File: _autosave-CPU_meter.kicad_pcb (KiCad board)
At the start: 4 copper layers, 25 parts, among them IC1 ATMEGA328P-P, SW1 SPST, U1 74HC595, U2 74HC595, U3 74HC595, U4 74HC595, U5 74HC595, U6 LM7805, Y1 16.00 MHz

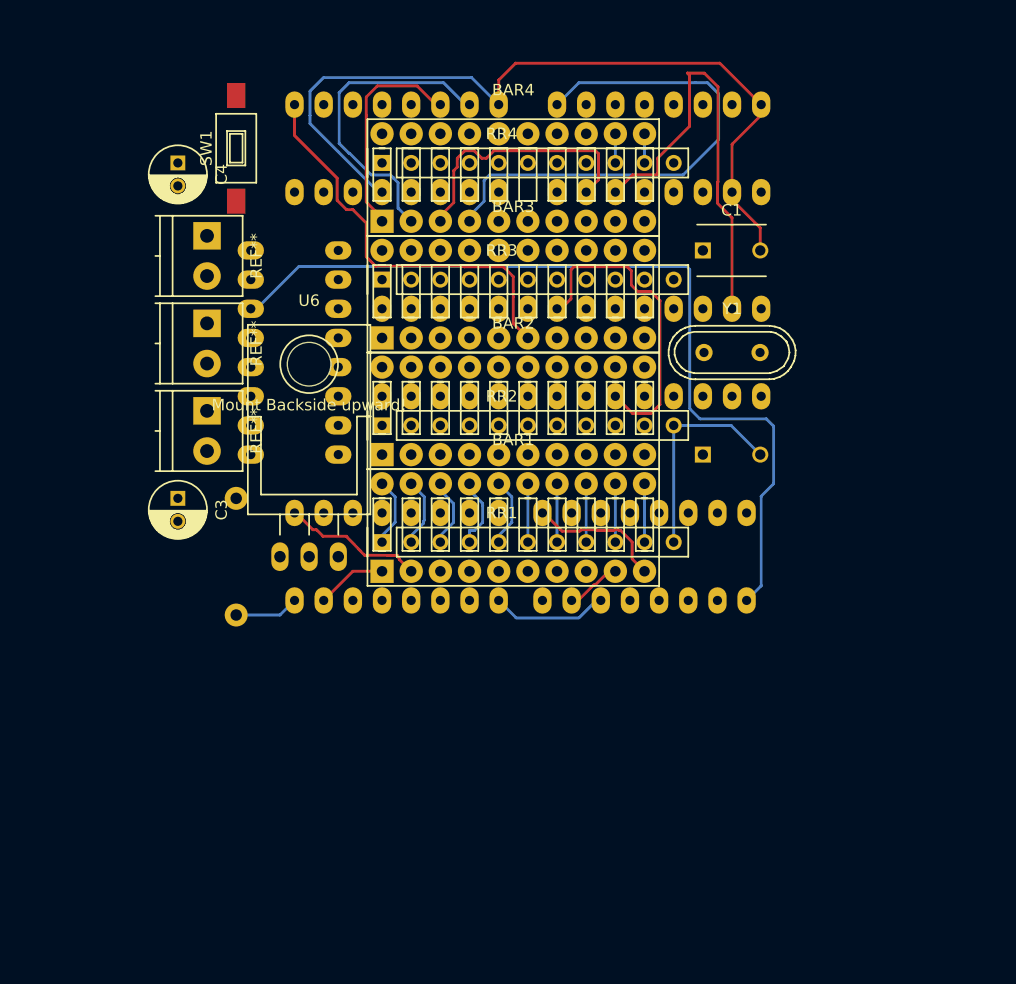
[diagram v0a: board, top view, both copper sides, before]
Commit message: PCB progress :)
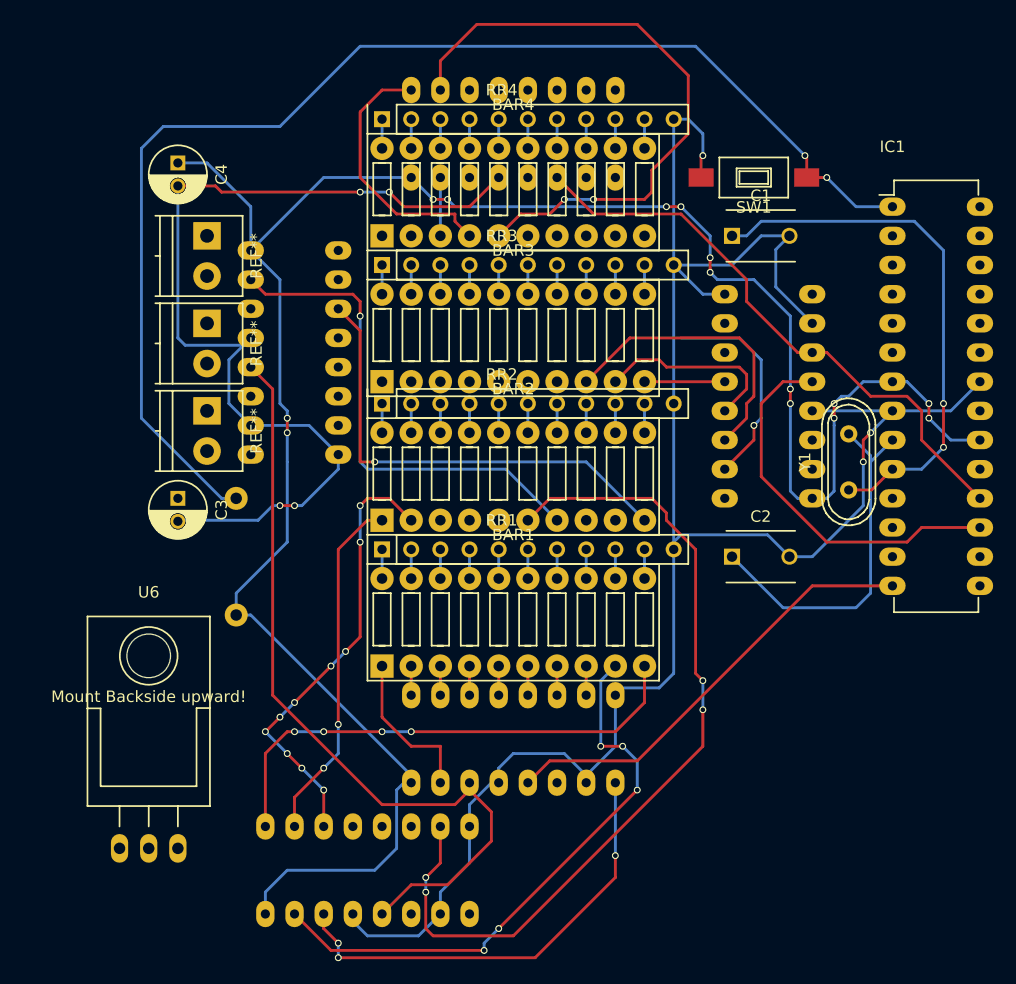
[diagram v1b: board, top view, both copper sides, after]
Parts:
- C2, IC1: moved to F.Cu
- moved U4 50.8 mm to (160.7, 147.3), turned to 0 degrees
- moved IC1 45.3 mm to (175.3, 121.9), turned to 0 degrees
- moved SW1 45.2 mm to (163.2, 119.4), turned to 180 degrees
- moved U2 36.4 mm to (120.7, 175.9)
- moved U6 29.0 mm to (110.5, 177.8)
- moved U1 18.8 mm to (133.3, 164.5)
- moved Y1 13.9 mm to (171.4, 144.1), turned to 90 degrees
- moved U5 12.8 mm to (133.3, 111.8)
- moved C2 9.25 mm to (161.3, 152.4)
- moved BAR1 8.25 mm to (142.2, 158.1)
- moved BAR2 5.72 mm to (142.2, 145.4)
- moved BAR3 3.81 mm to (142.2, 133.3)
- moved RR4 3.81 mm to (142.2, 114.3)
- moved C1 2.84 mm to (161.3, 124.5)
- moved RR2 1.91 mm to (142.2, 139.1)
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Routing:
- net GND: track 128.7 -> 258.1 mm, vias 0 -> 7
- net Net-(IC1-Pad1): track 0.00 -> 110.5 mm, vias 0 -> 2
- net Net-(IC1-Pad17): track 0.00 -> 102.5 mm
- net VCC: track 95.8 -> 189.5 mm, vias 0 -> 14
- net Net-(U2-Pad9): track 76.1 -> 0.00 mm
- net Net-(BAR2-Pad6): track 0.00 -> 75.7 mm, vias 0 -> 4
- net Net-(IC1-Pad18): track 0.00 -> 51.0 mm
- net Net-(BAR1-Pad9): track 4.86 -> 51.1 mm, vias 0 -> 5
- net Net-(BAR2-Pad7): track 0.00 -> 43.5 mm, vias 0 -> 1
- net Net-(BAR3-Pad10): track 50.2 -> 6.99 mm
- net Net-(BAR2-Pad10): track 0.00 -> 41.0 mm, vias 0 -> 1
- net Net-(BAR2-Pad2): track 0.00 -> 39.0 mm, vias 0 -> 10
- net Net-(IC1-Pad14): track 0.00 -> 38.9 mm
- net Net-(IC1-Pad13): track 37.4 -> 0.00 mm
- net Net-(C1-Pad1): track 9.84 -> 46.9 mm, vias 0 -> 2
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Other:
- copper layers 4 -> 2
